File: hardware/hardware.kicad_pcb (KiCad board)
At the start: 2 copper layers, 22 parts, among them J1 Screw_Terminal_01x02, J2 Screw_Terminal_01x02, J3 Screw_Terminal_01x02, K1 RM85-2011-35-1005, K2 RM85-2011-35-1005, Q1 BC337, Q2 BC337, U1 XIAO-ESP32-C6, U2 DS18B20

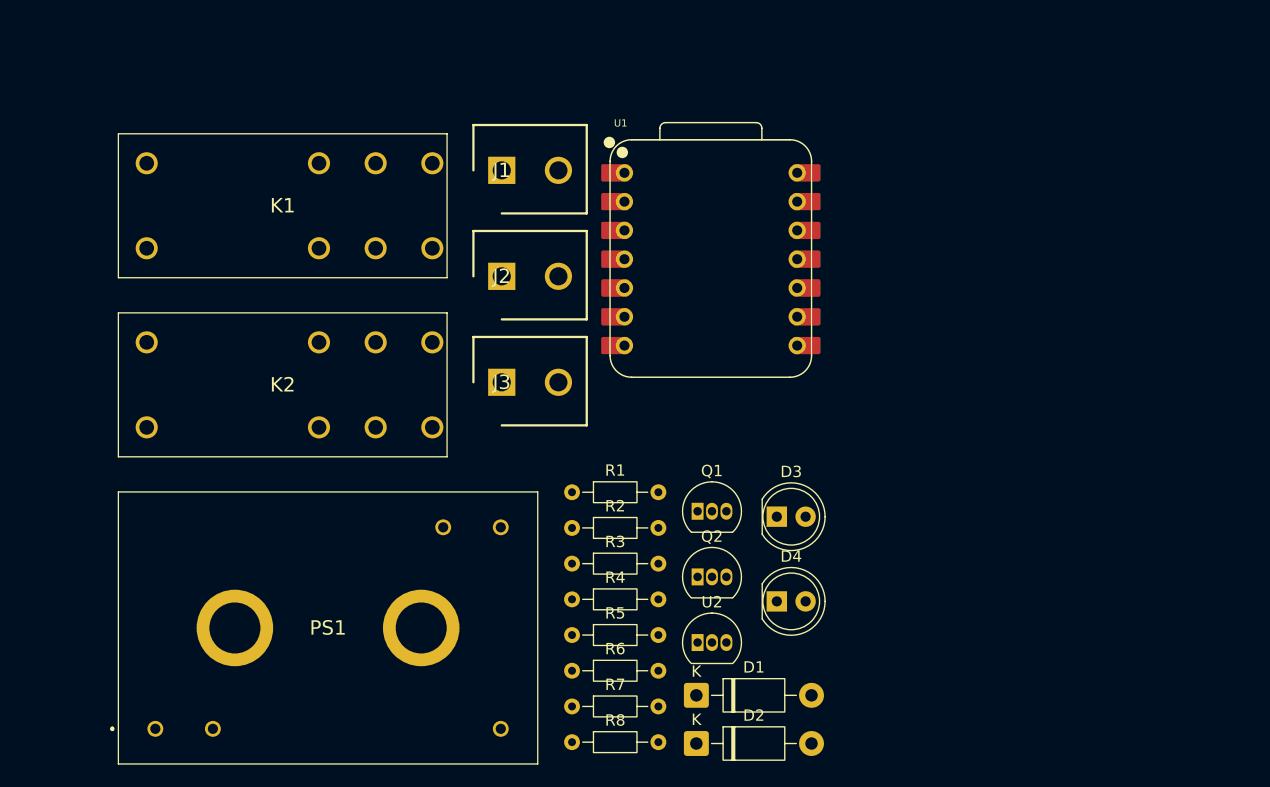
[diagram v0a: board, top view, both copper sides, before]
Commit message: Started working on PCB
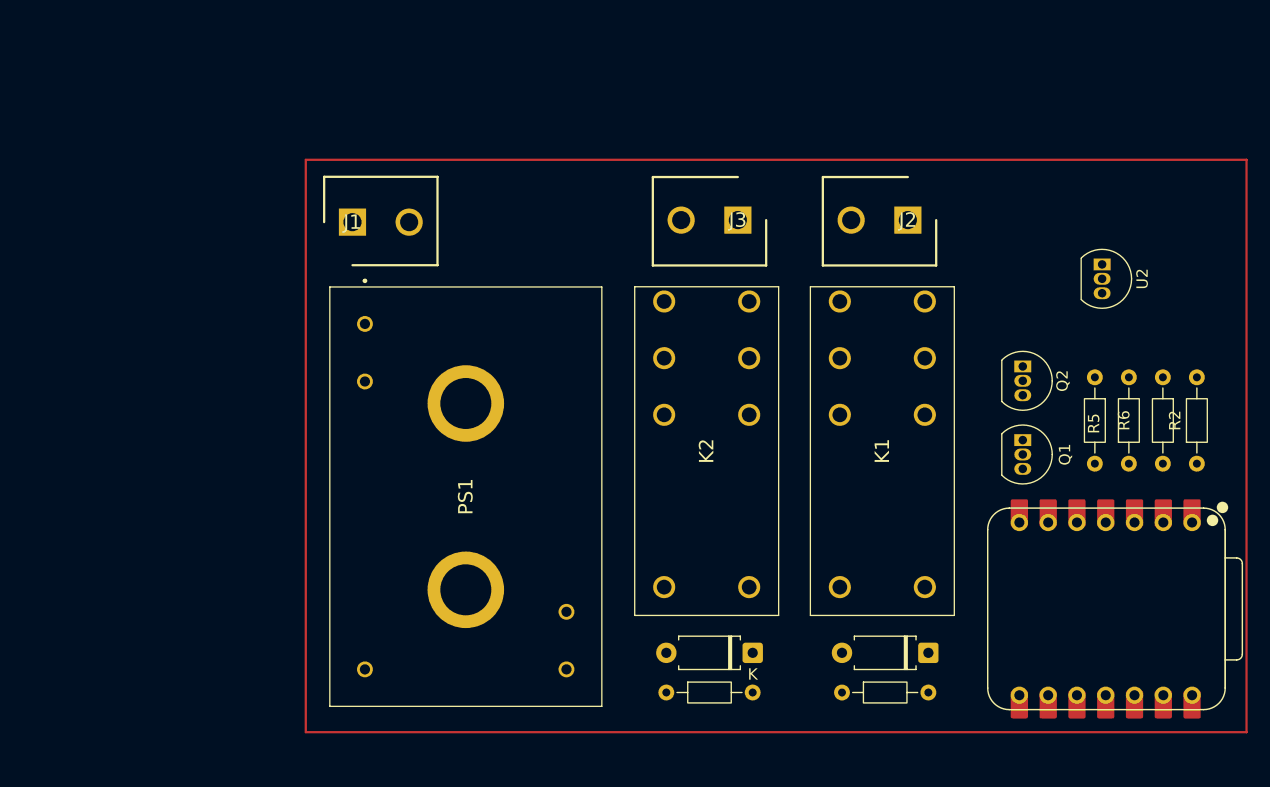
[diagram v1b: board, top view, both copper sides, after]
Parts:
- removed D3, D4: LED, LED_THT:LED_D5.0mm
- removed R7, R8: 100R, Resistor_THT:R_Axial_DIN0204_L3.6mm_D1.6mm_P7.62mm_Horizontal
- D1, D2: footprint Diode_THT:D_DO-41_SOD81_P10.16mm_Horizontal -> Diode_THT:D_A-405_P7.62mm_Horizontal
- moved R4 55.7 mm to (115.5, 46.2), turned to -90 degrees
- moved R2 55.4 mm to (118.5, 53.8), turned to 90 degrees
- moved R6 52.4 mm to (112.5, 53.8), turned to 90 degrees
- moved R5 51.4 mm to (109.5, 46.2), turned to -90 degrees
- moved K1 49.4 mm to (94.5, 44.5), turned to 90 degrees
- moved U2 48.9 mm to (110.1, 36.2), turned to -90 degrees
- moved U1 46.5 mm to (110.5, 66.7), turned to -90 degrees
- moved PS1 40.2 mm to (45.1, 41.5), turned to -90 degrees
- moved J2 36.2 mm to (93.0, 32.3), turned to 180 degrees
- moved Q2 34.2 mm to (103.1, 45.2), turned to -90 degrees
- moved K2 33.5 mm to (79.0, 44.5), turned to 90 degrees
- moved R1 29.7 mm to (87.2, 74.0)
- moved Q1 29.4 mm to (103.1, 51.7), turned to -90 degrees
- moved J3 25.3 mm to (78.0, 32.3), turned to 180 degrees
- moved D1 20.8 mm to (94.8, 70.5), turned to 180 degrees
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
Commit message: Improved PCB layout
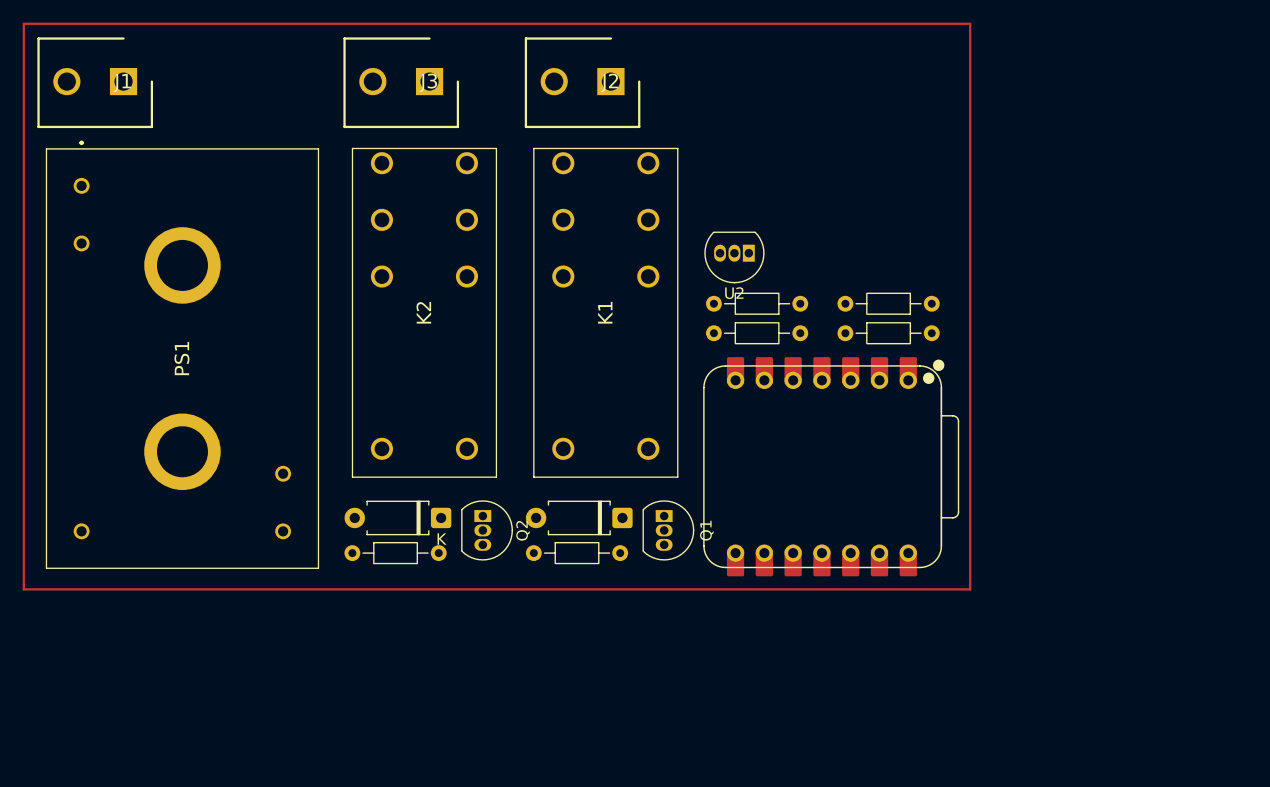
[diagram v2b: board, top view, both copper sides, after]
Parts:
- moved Q2 49.4 mm to (55.5, 58.4)
- moved R5 33.8 mm to (75.9, 42.3), turned to 0 degrees
- moved Q1 32.3 mm to (71.5, 58.4)
- moved R6 32.2 mm to (83.5, 39.7), turned to 180 degrees
- moved U2 31.2 mm to (79.0, 35.2), turned to 180 degrees
- moved R3 30.3 mm to (44.0, 61.7)
- moved D2 30.0 mm to (51.8, 58.6)
- moved R1 29.8 mm to (60.0, 61.7)
- moved J3 29.8 mm to (50.8, 20.1)
- moved D1 29.5 mm to (67.8, 58.6)
- moved J2 28.9 mm to (66.8, 20.1)
- moved R4 28.3 mm to (87.5, 42.3), turned to 0 degrees
- moved U1 28.0 mm to (85.4, 54.1)
- moved PS1 27.8 mm to (20.1, 29.3)
- moved K2 27.7 mm to (54.1, 32.3)
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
